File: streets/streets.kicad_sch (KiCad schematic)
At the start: 11 parts, among them J1 Barrel_Jack, J2 Conn_02x20_Odd_Even, J3 Conn_02x20_Odd_Even, J4 Conn_02x20_Odd_Even, J5 Conn_02x20_Odd_Even

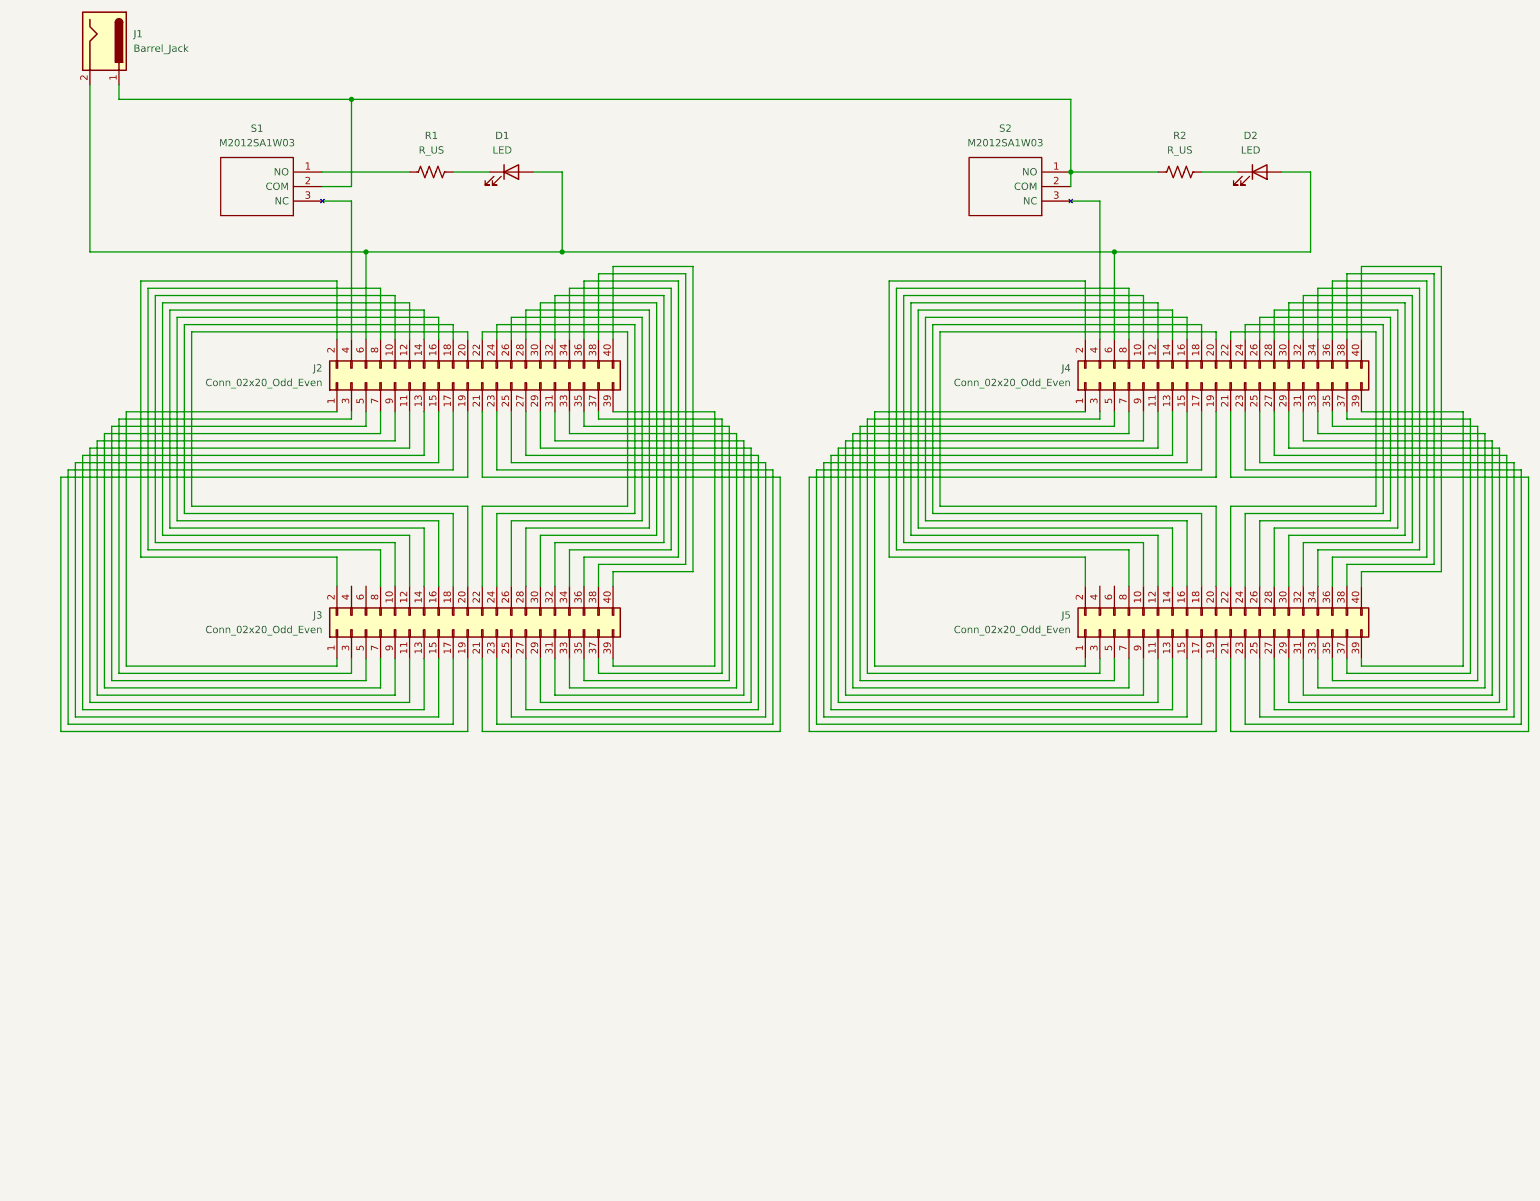
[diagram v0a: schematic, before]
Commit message: feat: refactor to use bus
Signed-off-by: Matt Gleich <git@mattglei.ch>
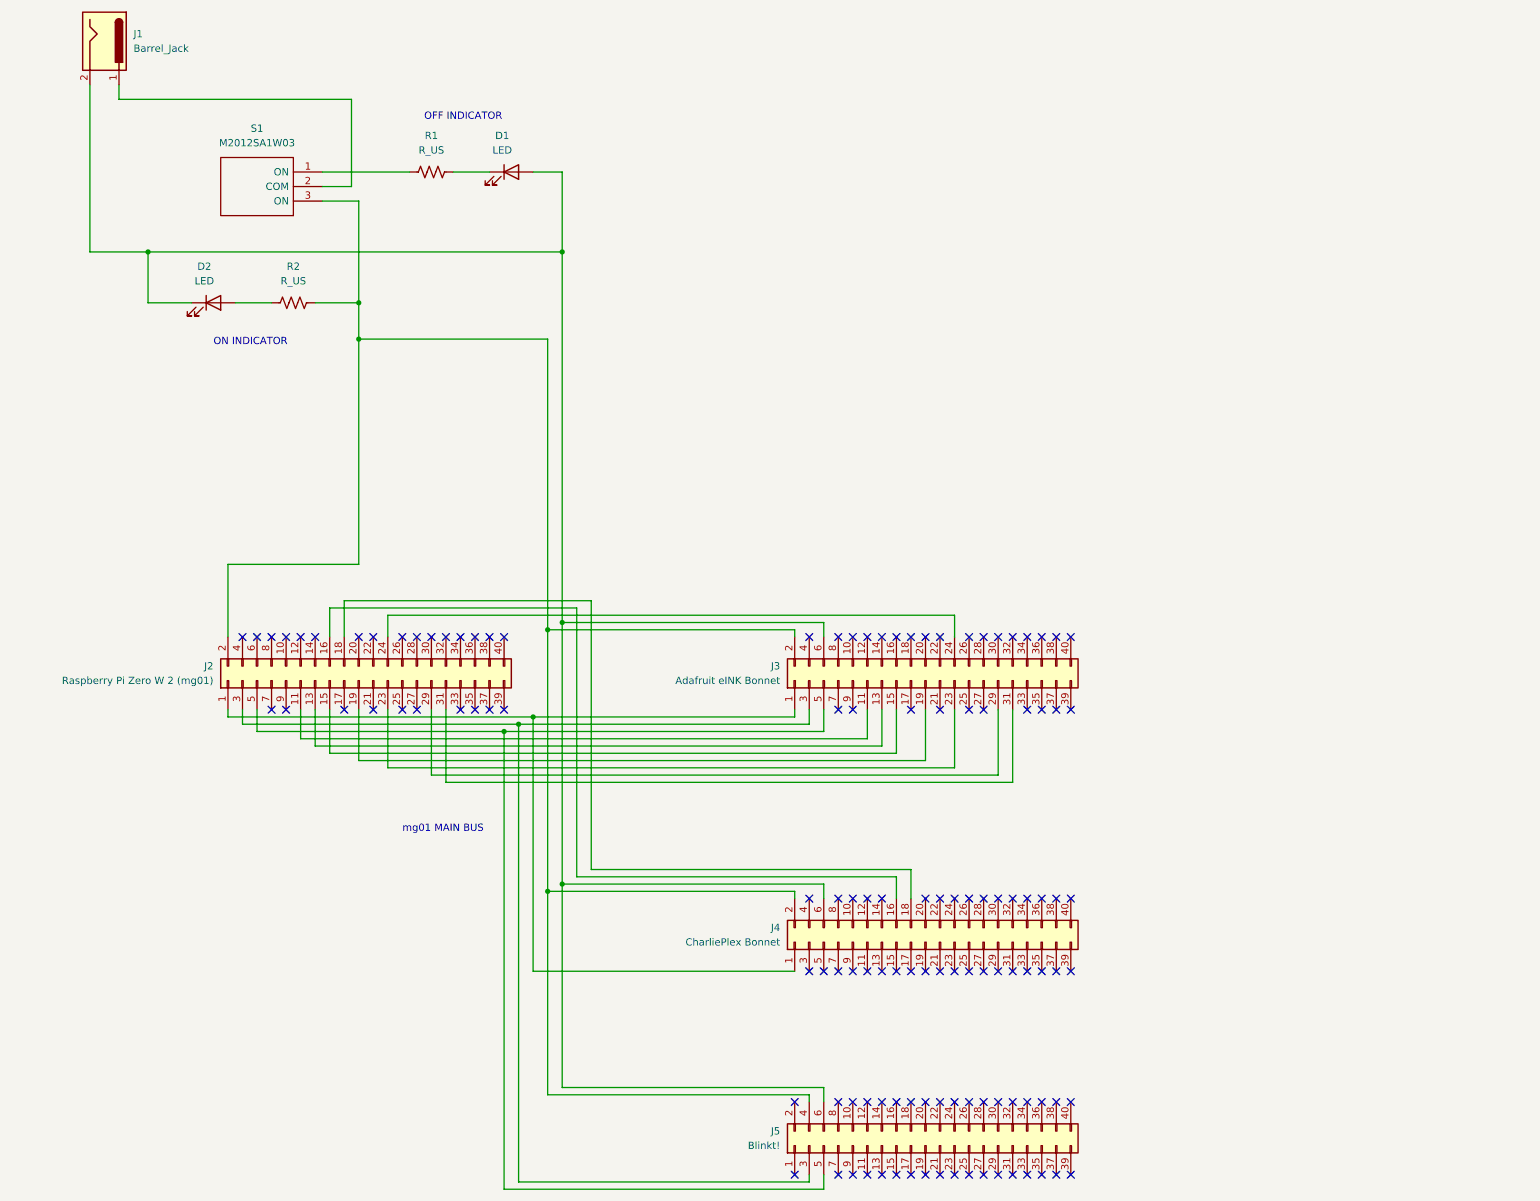
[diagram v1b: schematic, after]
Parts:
- removed S2: M2012SA1W03, M2012SA1W03, symbol M2012SA1W03:M2012SA1W03
- J2: value Conn_02x20_Odd_Even -> Raspberry Pi Zero W 2 (mg01)
- J3: value Conn_02x20_Odd_Even -> Adafruit eINK Bonnet
- J4: value Conn_02x20_Odd_Even -> CharliePlex Bonnet
- J5: value Conn_02x20_Odd_Even -> Blinkt!
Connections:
- net at D1.2 (A), J1.2, J4.6 (Pin_6): now also D2.1 (K), J3.6 (Pin_6), J5.6 (Pin_6); no longer D2.2 (A), J2.6 (Pin_6)
- net at J1.1, S1.2 (COM): no longer R2.1
- net at S1.3 (ON): now also J2.2 (Pin_2), J3.2 (Pin_2), J4.2 (Pin_2), J5.4 (Pin_4), R2.2; no longer J2.4 (Pin_4)
- net at J2.1 (Pin_1), J3.1 (Pin_1): now also J4.1 (Pin_1)
- net at J2.10 (Pin_10): no longer J3.10 (Pin_10)
- net at J2.12 (Pin_12): no longer J3.12 (Pin_12)
- net at J2.14 (Pin_14): no longer J3.14 (Pin_14)
- net at J2.16 (Pin_16): now also J4.16 (Pin_16); no longer J3.16 (Pin_16)
- net at J2.17 (Pin_17): no longer J3.17 (Pin_17)
- net at J2.18 (Pin_18): now also J4.18 (Pin_18); no longer J3.18 (Pin_18)
- net at J2.20 (Pin_20): no longer J3.20 (Pin_20)
- net at J2.21 (Pin_21): no longer J3.21 (Pin_21)
- net at J2.22 (Pin_22): no longer J3.22 (Pin_22)
- net at J2.25 (Pin_25): no longer J3.25 (Pin_25)
- net at J2.26 (Pin_26): no longer J3.26 (Pin_26)
- net at J2.27 (Pin_27): no longer J3.27 (Pin_27)
- net at J2.28 (Pin_28): no longer J3.28 (Pin_28)
- net at J2.3 (Pin_3), J3.3 (Pin_3): now also J5.3 (Pin_3)
- net at J2.30 (Pin_30): no longer J3.30 (Pin_30)
- net at J2.32 (Pin_32): no longer J3.32 (Pin_32)
- net at J2.33 (Pin_33): no longer J3.33 (Pin_33)
- net at J2.34 (Pin_34): no longer J3.34 (Pin_34)
- net at J2.35 (Pin_35): no longer J3.35 (Pin_35)
- net at J2.36 (Pin_36): no longer J3.36 (Pin_36)
- net at J2.37 (Pin_37): no longer J3.37 (Pin_37)
- net at J2.38 (Pin_38): no longer J3.38 (Pin_38)
- net at J2.39 (Pin_39): no longer J3.39 (Pin_39)
- net at J2.40 (Pin_40): no longer J3.40 (Pin_40)
- net at J2.5 (Pin_5), J3.5 (Pin_5): now also J5.5 (Pin_5)
- net at J2.7 (Pin_7): no longer J3.7 (Pin_7)
- net at J2.8 (Pin_8): no longer J3.8 (Pin_8)
- net at J2.9 (Pin_9): no longer J3.9 (Pin_9)
- net at J5.1 (Pin_1): no longer J4.1 (Pin_1)
- net at J4.10 (Pin_10): no longer J5.10 (Pin_10)
- net at J4.11 (Pin_11): no longer J5.11 (Pin_11)
- net at J4.12 (Pin_12): no longer J5.12 (Pin_12)
- net at J4.13 (Pin_13): no longer J5.13 (Pin_13)
- net at J4.14 (Pin_14): no longer J5.14 (Pin_14)
- net at J4.15 (Pin_15): no longer J5.15 (Pin_15)
- net at J5.16 (Pin_16): no longer J4.16 (Pin_16)
- net at J4.17 (Pin_17): no longer J5.17 (Pin_17)
- net at J5.18 (Pin_18): no longer J4.18 (Pin_18)
- net at J4.19 (Pin_19): no longer J5.19 (Pin_19)
- net at J5.2 (Pin_2): no longer J4.2 (Pin_2)
- net at J4.20 (Pin_20): no longer J5.20 (Pin_20)
- net at J4.21 (Pin_21): no longer J5.21 (Pin_21)
- net at J4.22 (Pin_22): no longer J5.22 (Pin_22)
- net at J4.23 (Pin_23): no longer J5.23 (Pin_23)
- net at J4.24 (Pin_24): no longer J5.24 (Pin_24)
- net at J4.25 (Pin_25): no longer J5.25 (Pin_25)
- net at J4.26 (Pin_26): no longer J5.26 (Pin_26)
- net at J4.27 (Pin_27): no longer J5.27 (Pin_27)
- net at J4.28 (Pin_28): no longer J5.28 (Pin_28)
- net at J4.29 (Pin_29): no longer J5.29 (Pin_29)
- net at J4.3 (Pin_3): no longer J5.3 (Pin_3)
- net at J4.30 (Pin_30): no longer J5.30 (Pin_30)
- net at J4.31 (Pin_31): no longer J5.31 (Pin_31)
- net at J4.32 (Pin_32): no longer J5.32 (Pin_32)
- net at J4.33 (Pin_33): no longer J5.33 (Pin_33)
- net at J4.34 (Pin_34): no longer J5.34 (Pin_34)
- net at J4.35 (Pin_35): no longer J5.35 (Pin_35)
- net at J4.36 (Pin_36): no longer J5.36 (Pin_36)
- net at J4.37 (Pin_37): no longer J5.37 (Pin_37)
- net at J4.38 (Pin_38): no longer J5.38 (Pin_38)
- net at J4.39 (Pin_39): no longer J5.39 (Pin_39)
- net at J4.40 (Pin_40): no longer J5.40 (Pin_40)
- net at J4.5 (Pin_5): no longer J5.5 (Pin_5)
- net at J4.7 (Pin_7): no longer J5.7 (Pin_7)
- net at J4.8 (Pin_8): no longer J5.8 (Pin_8)
- net at J4.9 (Pin_9): no longer J5.9 (Pin_9)
- new net: D2.2 (A), R2.1
- no-connect marks 0 -> 124
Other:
- note added: "OFF INDICATOR"
- note added: "ON INDICATOR"
- note added: "mg01 MAIN BUS"
